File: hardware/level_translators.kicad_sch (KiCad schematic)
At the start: 30 parts, among them U10 UM3304, U11 UM3304, U12 UM3304, U13 UM3304, U14 UM3304, U15 UM3304

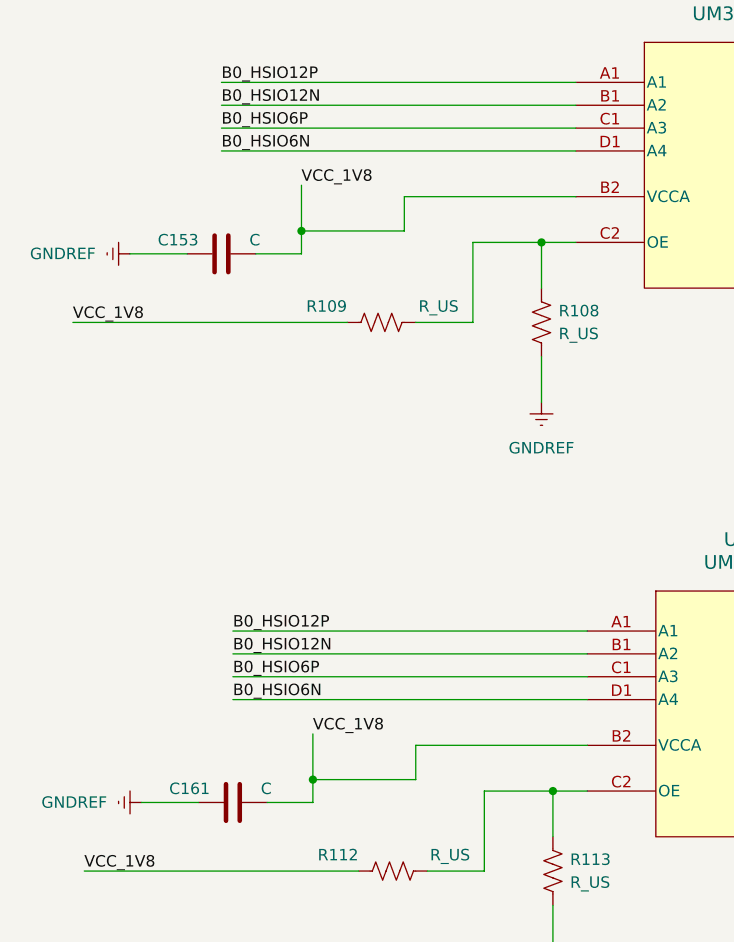
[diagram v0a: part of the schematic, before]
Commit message: updated hardware
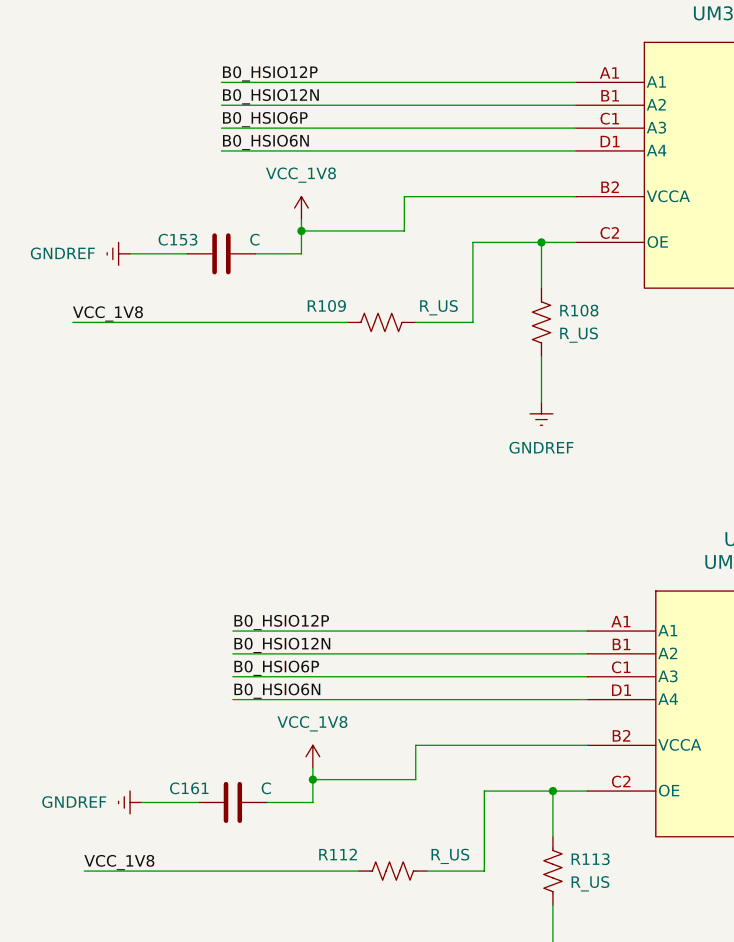
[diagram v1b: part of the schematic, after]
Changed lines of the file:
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@@
+	)
+	(junction
+		(at 82.55 74.93)
+		(diameter 0)
+		(color 0 0 0 0)
 	)
 	(junction
@@
 	)
 	(junction
-		(at 82.55 74.93)
-		(diameter 0)
-		(color 0 0 0 0)
-	)
-	(junction
 		(at 177.8 135.89)
 		(diameter 0)
@@
 	(wire
 		(pts
-			(xy 83.82 130.81) (xy 83.82 135.89)
-		)
-		(stroke
-			(width 0)
-			(type default)
-		)
-	)
-	(wire
-		(pts
 			(xy 245.11 60.96) (xy 284.48 60.96)
 		)
@@
 	(wire
 		(pts
+			(xy 83.82 134.62) (xy 83.82 135.89)
+		)
+		(stroke
+			(width 0)
+			(type default)
+		)
+	)
+	(wire
+		(pts
 			(xy 97.79 203.2) (xy 104.14 203.2)
 		)
@@
 	(wire
 		(pts
-			(xy 82.55 69.85) (xy 82.55 74.93)
+			(xy 82.55 73.66) (xy 82.55 74.93)
 		)
 		(stroke
@@
 		)
 	)
-	(label "VCC_1V8"
-		(at 83.82 130.81 0)
-		(effects
-			(font
-				(size 1.27 1.27)
-			)
-			(justify left bottom)
-		)
-	)
 	(label "VCC_3V3"
 		(at 346.71 187.96 180)
@@
 	(label "VCC_1V8"
 		(at 254 130.81 0)
-		(effects
-			(font
-				(size 1.27 1.27)
-			)
-			(justify left bottom)
-		)
-	)
-	(label "VCC_1V8"
-		(at 82.55 69.85 0)
 		(effects
 			(font
@@
 				(path "/ffb442c5-ffd1-4efa-a6fc-c35cfd4b76ad"
 					(reference "R110")
+					(unit 1)
+				)
+			)
+		)
+	)
+	(symbol
+		(lib_id "power:VDD")
+		(at 82.55 73.66 0)
+		(unit 1)
+		(body_style 1)
+		(exclude_from_sim no)
+		(in_bom yes)
+		(on_board yes)
+		(in_pos_files yes)
+		(dnp no)
+		(fields_autoplaced yes)
+		(property "Reference" "#PWR0215"
+			(at 82.55 77.47 0)
+			(hide yes)
+			(show_name no)
+			(do_not_autoplace no)
+			(effects
+				(font
+					(size 1.27 1.27)
+				)
+			)
+		)
+		(property "Value" "VCC_1V8"
+			(at 82.55 68.58 0)
+			(show_name no)
+			(do_not_autoplace no)
+			(effects
+				(font
+					(size 1.27 1.27)
+				)
+			)
+		)
+		(property "Footprint" ""
+			(at 82.55 73.66 0)
+			(hide yes)
+			(show_name no)
+			(do_not_autoplace no)
+			(effects
+				(font
+					(size 1.27 1.27)
+				)
+			)
+		)
+		(property "Datasheet" ""
+			(at 82.55 73.66 0)
+			(hide yes)
+			(show_name no)
+			(do_not_autoplace no)
+			(effects
+				(font
+					(size 1.27 1.27)
+				)
+			)
+		)
+		(property "Description" "Power symbol creates a global label with name \"VDD\""
+			(at 82.55 73.66 0)
+			(hide yes)
+			(show_name no)
+			(do_not_autoplace no)
+			(effects
+				(font
+					(size 1.27 1.27)
+				)
+			)
+		)
+		(pin "1"
+		)
+		(instances
+			(project "RO-Instrument"
+				(path "/ffb442c5-ffd1-4efa-a6fc-c35cfd4b76ad"
+					(reference "#PWR0215")
 					(unit 1)
 				)
@@
 					(unit 1)
 				)
+			)
+		)
+	)
+	(symbol
+		(lib_id "power:VDD")
+		(at 83.82 134.62 0)
+		(unit 1)
+		(body_style 1)
+		(exclude_from_sim no)
+		(in_bom yes)
+		(on_board yes)
+		(in_pos_files yes)
+		(dnp no)
+		(fields_autoplaced yes)
+		(property "Reference" "#PWR0214"
+			(at 83.82 138.43 0)
+			(hide yes)
+			(show_name no)
+			(do_not_autoplace no)
+			(effects
+				(font
+					(size 1.27 1.27)
+				)
+			)
+		)
+		(property "Value" "VCC_1V8"
+			(at 83.82 129.54 0)
+			(show_name no)
+			(do_not_autoplace no)
+			(effects
+				(font
+					(size 1.27 1.27)
+				)
+			)
+		)
+		(property "Footprint" ""
+			(at 83.82 134.62 0)
+			(hide yes)
+			(show_name no)
+			(do_not_autoplace no)
+			(effects
+				(font
+					(size 1.27 1.27)
+				)
+			)
+		)
+		(property "Datasheet" ""
+			(at 83.82 134.62 0)
+			(hide yes)
+			(show_name no)
+			(do_not_autoplace no)
+			(effects
+				(font
+					(size 1.27 1.27)
+				)
+			)
+		)
+		(property "Description" "Power symbol creates a global label with name \"VDD\""
+			(at 83.82 134.62 0)
+			(hide yes)
+			(show_name no)
+			(do_not_autoplace no)
+			(effects
+				(font
+					(size 1.27 1.27)
+				)
+			)
+		)
+		(pin "1"
+		)
+		(instances
+			(project "RO-Instrument"
+				(path "/ffb442c5-ffd1-4efa-a6fc-c35cfd4b76ad"
+					(reference "#PWR0214")
+					(unit 1)
+				)
